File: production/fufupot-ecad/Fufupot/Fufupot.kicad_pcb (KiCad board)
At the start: 2 copper layers, 6 parts, among them U2 ATMEGA328P-PN

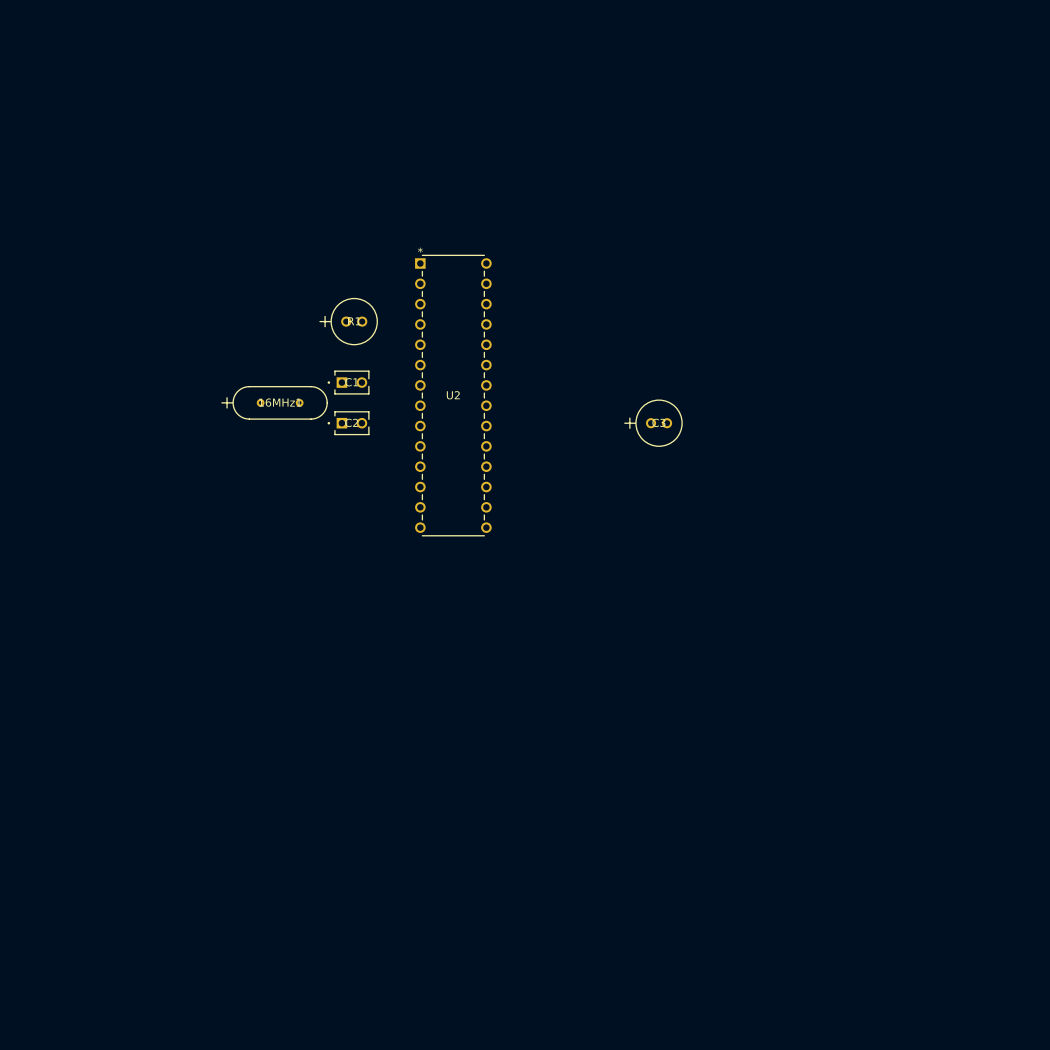
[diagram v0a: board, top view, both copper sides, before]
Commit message: Updates unfinished
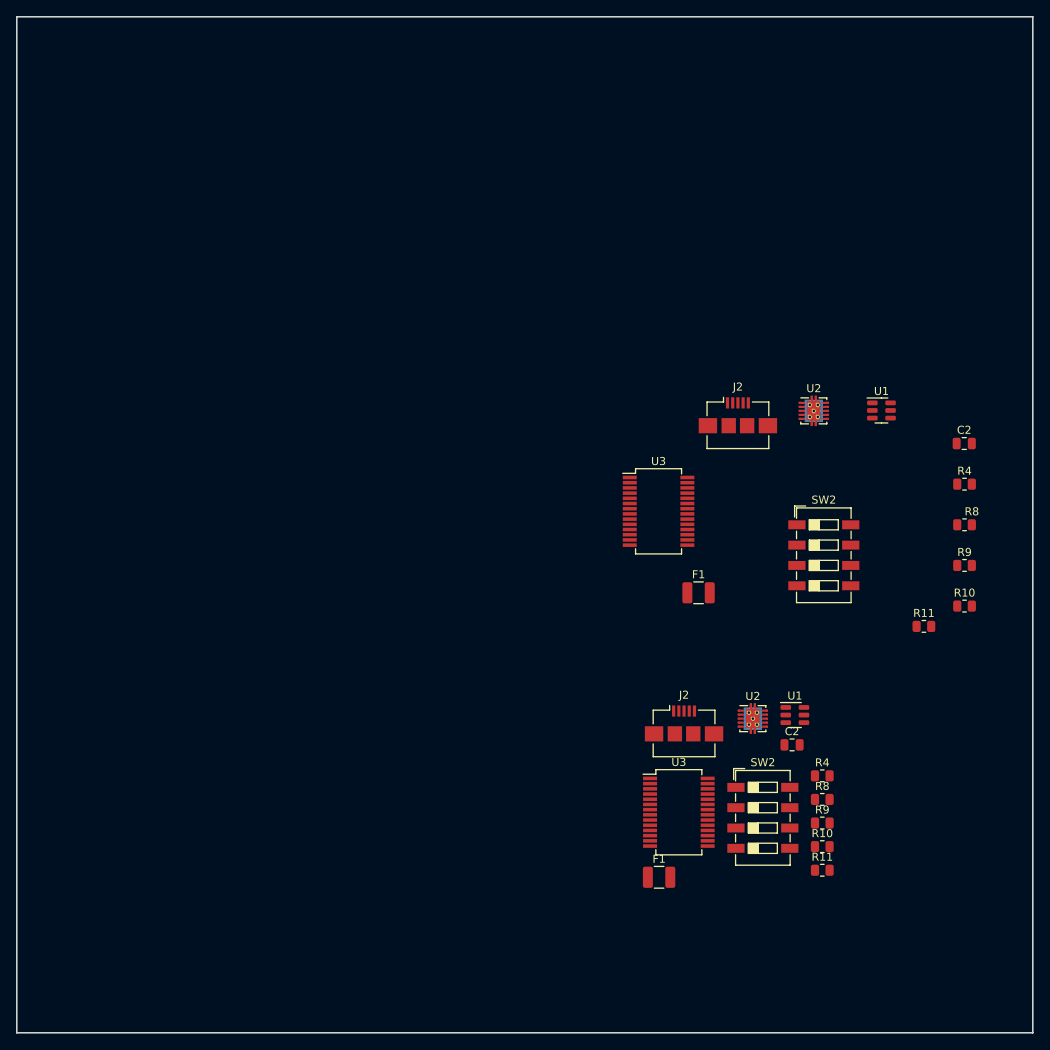
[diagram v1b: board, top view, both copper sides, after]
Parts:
- removed 16MHz1: Crystal, 16 MHz Xtal Osc:XTAL_ABL-16_ABR
- removed C1: 22pF, 22 pF Cap:CAP_K-SERIES_15-L2_VIS
- removed the C2 at (86.4, 86.4)
- removed C3: 10uF, 10 uF Cap:CAP_YX_5X11_RUB
- removed R1: 10k, 10K Ohm:CAP_YX_5X11_RUB
- removed the U2 at (96.2, 66.4)
- added C2: 100n, Capacitor_SMD:C_0805_2012Metric, F.Cu at (142.6, 126.6)
- added C2: 100n, Capacitor_SMD:C_0805_2012Metric, F.Cu at (164.2, 88.9)
- added F1: 500mA, Fuse:Fuse_1210_3225Metric, F.Cu at (130.9, 107.6)
- added F1: 500mA, Fuse:Fuse_1210_3225Metric, F.Cu at (126.0, 143.1)
- added J2: USB_B, Connector_USB:USB_Micro-B_Amphenol_10104110_Horizontal, F.Cu at (129.1, 123.9)
- added J2: USB_B, Connector_USB:USB_Micro-B_Amphenol_10104110_Horizontal, F.Cu at (135.9, 85.4)
- added R10: 1k, Resistor_SMD:R_0805_2012Metric, F.Cu at (164.2, 109.2)
- added R10: 1k, Resistor_SMD:R_0805_2012Metric, F.Cu at (146.4, 139.3)
- added R11: 1k, Resistor_SMD:R_0805_2012Metric, F.Cu at (159.1, 111.8)
- added R11: 1k, Resistor_SMD:R_0805_2012Metric, F.Cu at (146.4, 142.2)
- added R4: 10k, Resistor_SMD:R_0805_2012Metric, F.Cu at (164.2, 94.0)
- added R4: 10k, Resistor_SMD:R_0805_2012Metric, F.Cu at (146.4, 130.4)
- added R8: 1k, Resistor_SMD:R_0805_2012Metric, F.Cu at (164.2, 99.1)
- added R8: 1k, Resistor_SMD:R_0805_2012Metric, F.Cu at (146.4, 133.4)
- added R9: 1k, Resistor_SMD:R_0805_2012Metric, F.Cu at (164.2, 104.1)
- added R9: 1k, Resistor_SMD:R_0805_2012Metric, F.Cu at (146.4, 136.3)
- added SW2: SW_Push, Button_Switch_SMD:SW_DIP_SPSTx04_Slide_6.7x11.72mm_W6.73mm_P2.54mm_LowProfile_JPin, F.Cu at (139.0, 135.7)
- added SW2: SW_Push, Button_Switch_SMD:SW_DIP_SPSTx04_Slide_6.7x11.72mm_W6.73mm_P2.54mm_LowProfile_JPin, F.Cu at (146.6, 102.9)
- added U1: USBLC6-2SC6, Package_TO_SOT_SMD:SOT-23-6, F.Cu at (143.0, 122.8)
- added U1: USBLC6-2SC6, Package_TO_SOT_SMD:SOT-23-6, F.Cu at (153.8, 84.8)
- added U2: LM5165DRC, Package_SON:Texas_S-PVSON-N10_ThermalVias, F.Cu at (145.3, 84.8)
- added U2: LM5165DRC, Package_SON:Texas_S-PVSON-N10_ThermalVias, F.Cu at (137.7, 123.3)
- added U3: FT232RL, Package_SO:SSOP-28_5.3x10.2mm_P0.65mm, F.Cu at (128.5, 135.0)
- added U3: FT232RL, Package_SO:SSOP-28_5.3x10.2mm_P0.65mm, F.Cu at (125.9, 97.4)
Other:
- board outline added: 127 x 127 mm
- copper layers 2 -> 4
